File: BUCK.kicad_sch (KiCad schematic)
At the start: 11 parts, among them U2 TPS562200

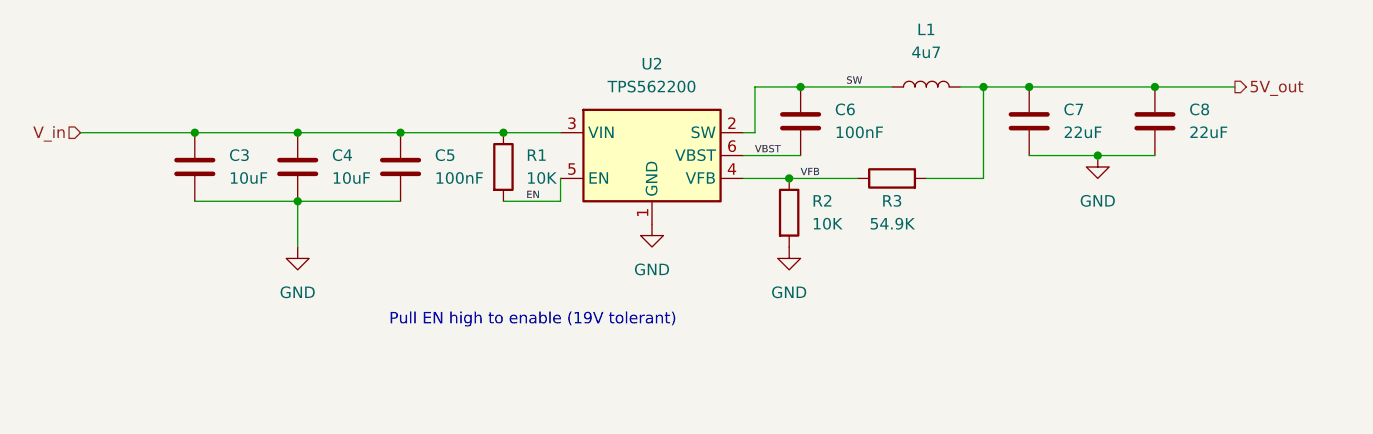
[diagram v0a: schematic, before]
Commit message: Updated subsheets
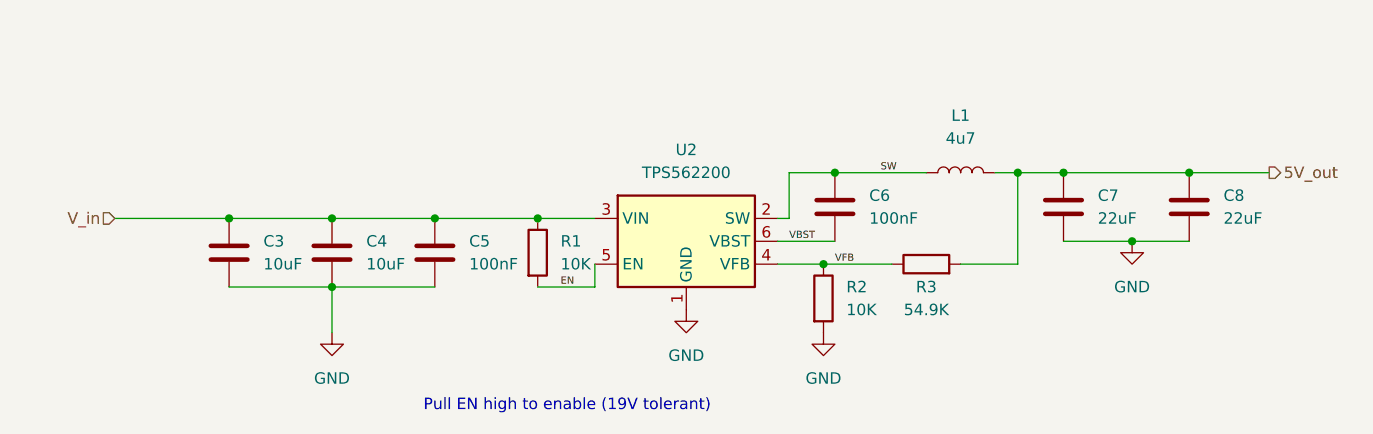
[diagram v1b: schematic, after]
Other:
- moved on the sheet: C3, C4, C5, C6, C7, C8, L1, R1, R2, R3, U2
